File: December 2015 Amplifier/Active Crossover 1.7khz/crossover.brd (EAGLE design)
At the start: 58.1 x 36.8 mm, 47 parts

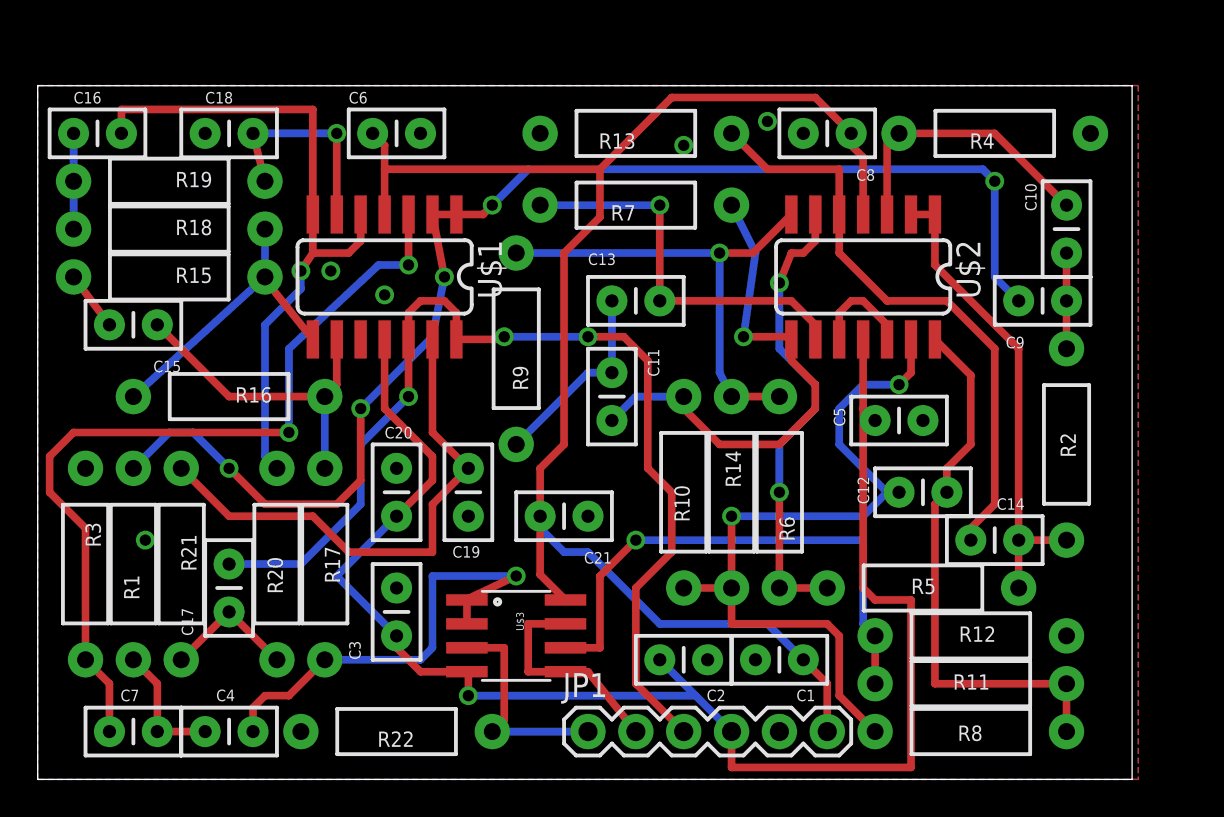
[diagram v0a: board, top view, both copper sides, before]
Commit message: Not Quite sure what is different, but there are the new files. :P
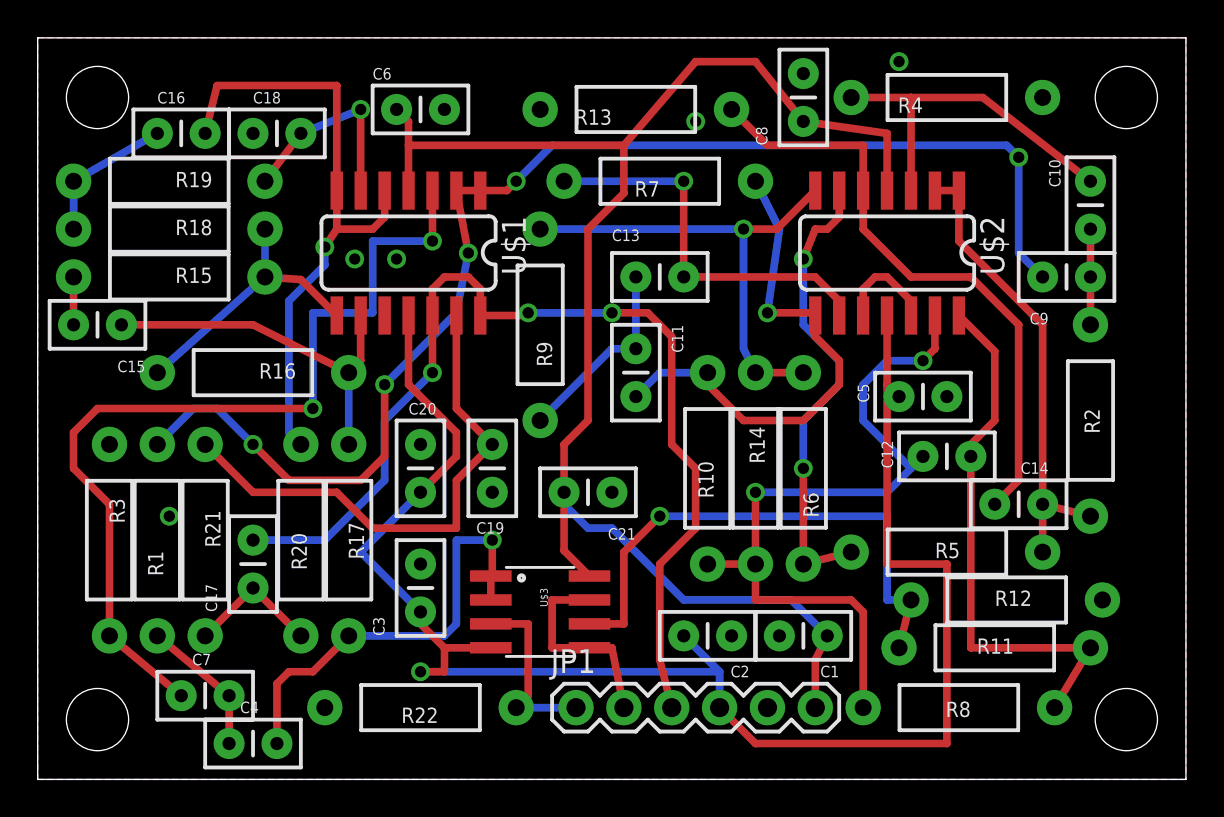
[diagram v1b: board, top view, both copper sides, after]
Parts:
- added U$4, U$5, U$6, U$7: (no value), SparkFun-Electromechanical:STAND-OFF
- moved C16 4.44 mm to (6.35, 34.3)
- moved C7 4.26 mm to (10.2, 4.45)
- moved R4 3.18 mm to (48.3, 36.2)
- moved R12 2.69 mm to (51.4, 9.53)
- moved C8 2.62 mm to (40.6, 34.9), turned to 90 degrees
- moved C18 2.54 mm to (11.4, 34.3)
- moved C14 2.29 mm to (53.3, 14.6)
- moved C12 2.29 mm to (47.0, 17.1)
- moved R11 2.29 mm to (50.8, 6.99)
- moved R5 2.29 mm to (48.3, 12.1)
- moved C15 1.90 mm to (4.45, 24.1)
- moved C9 1.80 mm to (53.3, 26.7)
- moved R10 1.80 mm to (35.6, 16.5)
- moved R14 1.80 mm to (38.1, 16.5)
- moved R6 1.80 mm to (40.6, 16.5)
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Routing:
- net VEE: track 81.1 -> 87.9 mm
- net N$12: track 15.4 -> 19.2 mm
- net N$1: track 44.4 -> 47.7 mm
- net N$33: track 5.08 -> 7.66 mm
- net N$35: track 35.9 -> 33.5 mm
- net N$29: track 17.6 -> 19.8 mm
- net INPUT: track 11.8 -> 9.86 mm
- net N$31: track 16.2 -> 14.8 mm
- net N$42: track 24.5 -> 23.6 mm
- net L_OUT: track 56.8 -> 55.8 mm
- net H_OUT: track 11.8 -> 10.9 mm
- net N$20: track 32.0 -> 32.6 mm
- net N$30: track 3.18 -> 2.54 mm
- net N$3: track 6.88 -> 7.50 mm
- net N$21: track 25.5 -> 24.9 mm
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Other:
- board size 58.1 x 36.8 mm -> 60.9 x 39.4 mm
